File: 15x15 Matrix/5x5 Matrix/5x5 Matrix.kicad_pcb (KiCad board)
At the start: 2 copper layers, 127.8 x 152.5 mm, 111 parts, among them J1 Conn_01x02, SW1 SWP, SW10 SWP, SW11 SWP, SW12 SWP, SW13 SWP, SW14 SWP, SW15 SWP, SW16 SWP, SW17 SWP, SW18 SWP, SW19 SWP, SW2 SWP, SW20 SWP, SW21 SWP, SW22 SWP, SW23 SWP, SW24 SWP, SW25 SWP, SW3 SWP, SW4 SWP, SW5 SWP, SW6 SWP, SW7 SWP, SW8 SWP, SW9 SWP, U1 MCP23017-E/SO, U2 74AHCT1G125

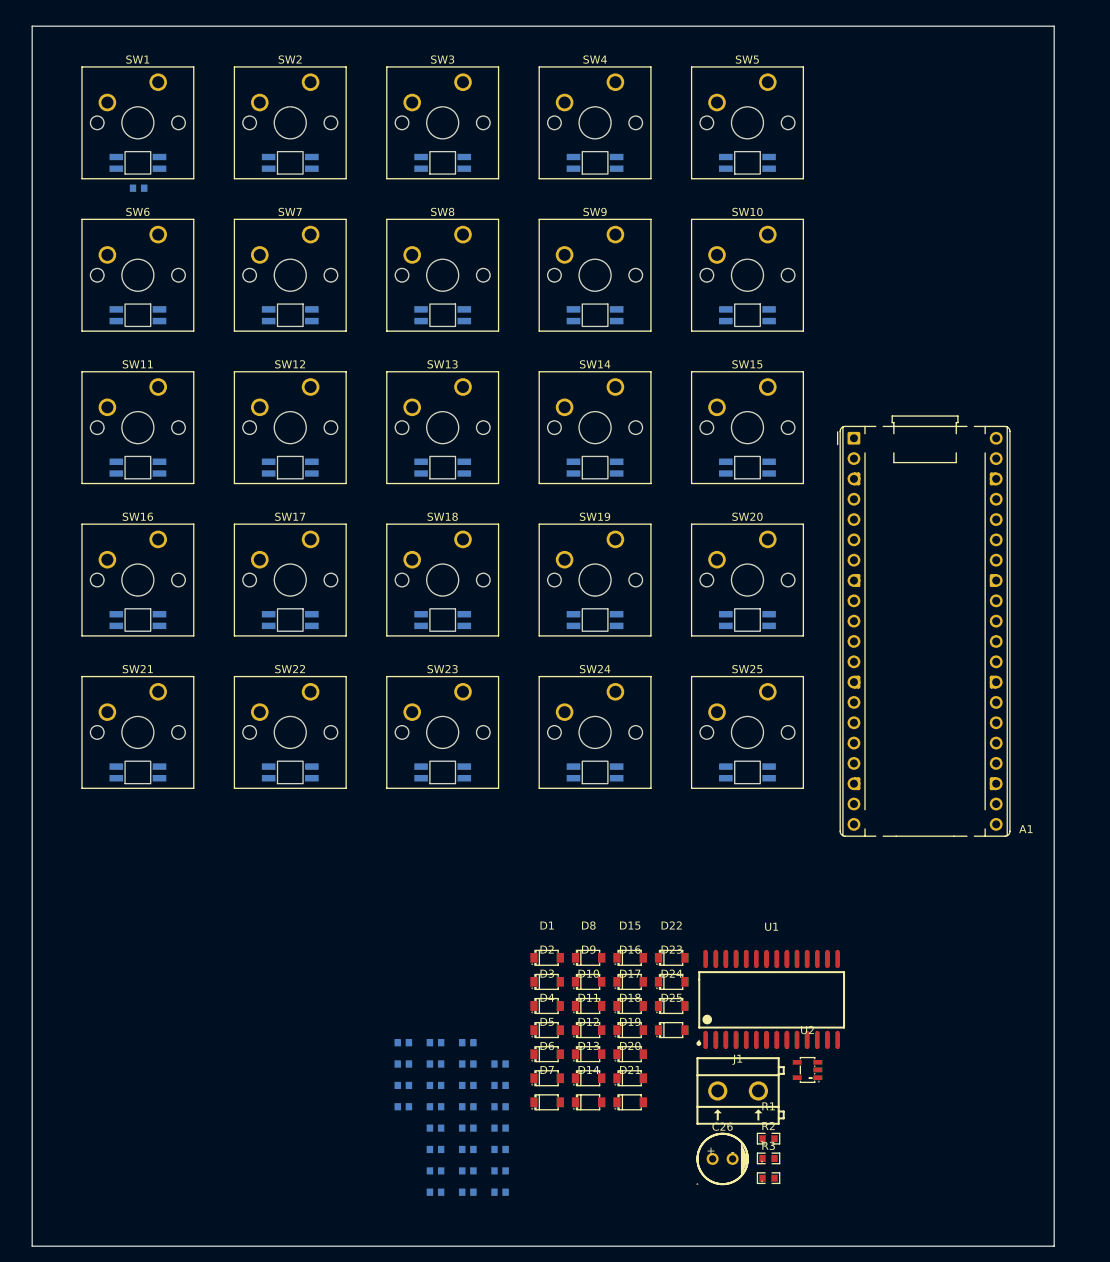
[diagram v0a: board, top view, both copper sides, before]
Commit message: 5x5 Ready for 1 sided printing
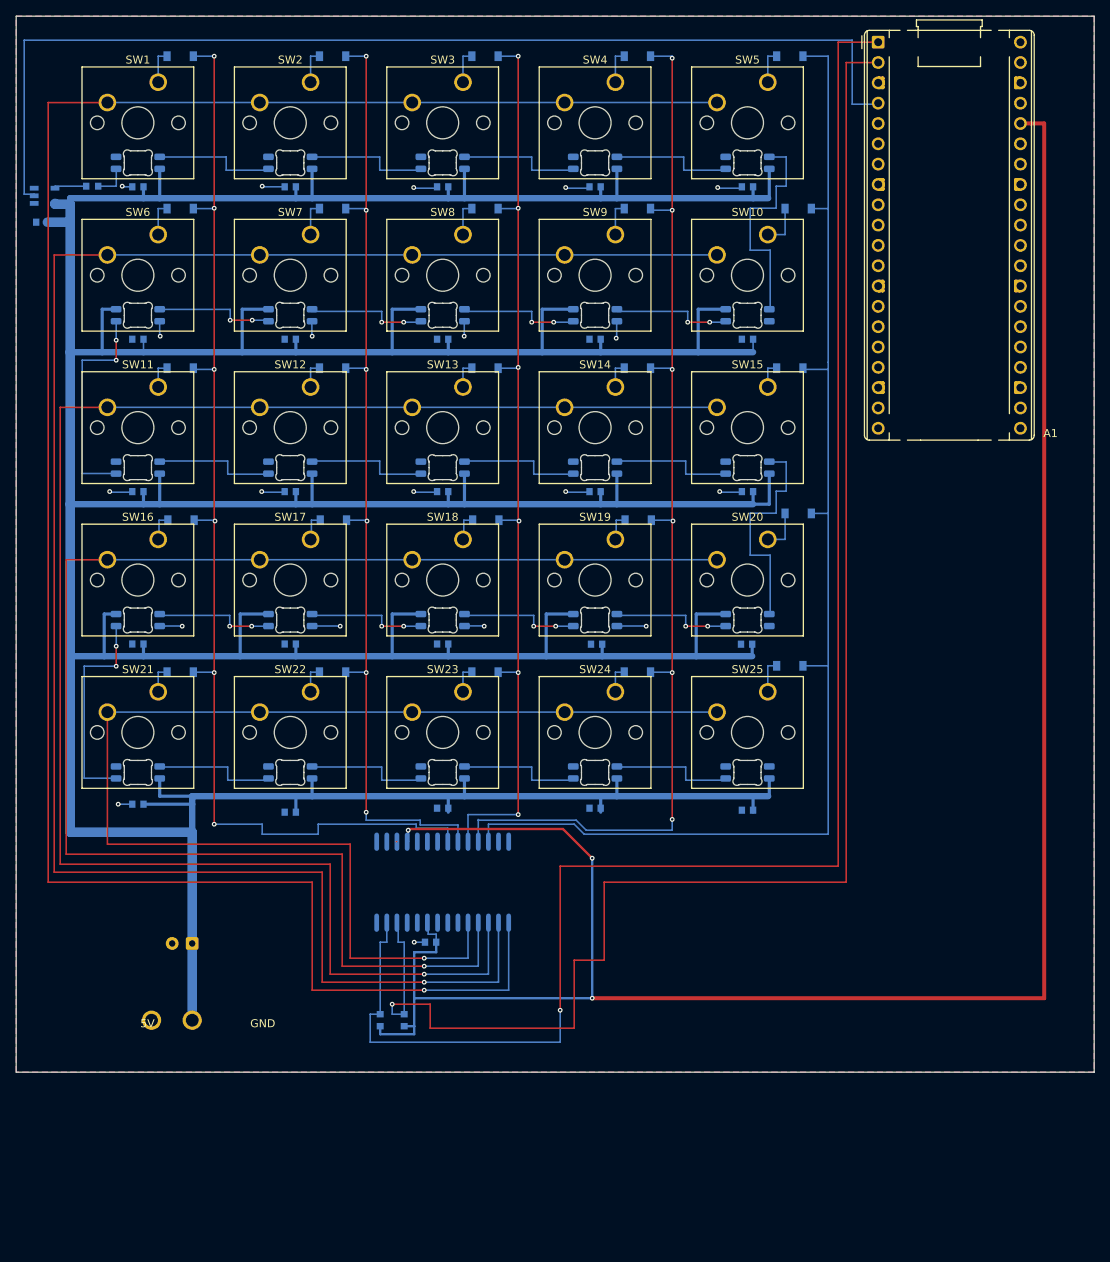
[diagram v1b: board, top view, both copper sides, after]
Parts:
- removed CPI1: 100nF, footprints:C14663_C0603
- C26: footprint footprints:C49304896_CAP-TH_BD6_3-P2_50-D0_5-FD -> Capacitor_THT:CP_Radial_D6.3mm_P2.50mm; moved to B.Cu
- D1, D10, D11, D12, D13, D14, D15, D16, D17, D18, D19, D2, D20, D21, D22, D23, D24, D25, D3, D4, D5, D6, D7, D8, D9, J1, R1, R2, R3, U1, U2: moved to B.Cu
- D26, D27, D28, D29, D30, D31, D32, D33, D34, D35, D36, D37, D38, D39, D40, D41, D42, D43, D44, D45, D46, D47, D48, D49, D50: footprint footprints:C5149201_LED-SMD_4P-L3_2-W2_8-LS5_9_SK6812MINI-E -> LED_SMD:LED_SK6812MINI-E_3.2x2.8mm_P1.5mm_ReverseMount
- moved R3 150.1 mm to (21.8, 43.0), turned to 180 degrees
- moved U2 145.0 mm to (15.8, 44.2), turned to 180 degrees
- moved D5 128.4 mm to (109.0, 26.8), turned to 180 degrees
- moved D4 122.3 mm to (89.9, 26.8), turned to 180 degrees
- moved D1 121.7 mm to (32.8, 26.8), turned to 180 degrees
- moved C5 121.7 mm to (103.7, 43.1)
- moved D3 119.0 mm to (70.8, 26.8), turned to 180 degrees
- moved D2 118.8 mm to (51.8, 26.8), turned to 180 degrees
- moved D6 118.0 mm to (32.8, 45.8), turned to 180 degrees
- moved C4 115.6 mm to (84.6, 43.1)
- moved D7 114.9 mm to (51.8, 45.8), turned to 180 degrees
- moved C27 114.5 mm to (15.4, 47.5), turned to 0 degrees
- moved C2 112.7 mm to (46.5, 43.1)
- moved C3 112.5 mm to (65.6, 43.1)
- moved C8 106.9 mm to (65.6, 62.1)
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- renumbered CPI2 to C28
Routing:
- net /5V: track 0.00 -> 727.9 mm
- net /ROW0: track 0.00 -> 260.6 mm, vias 0 -> 1
- net /3V3: track 0.00 -> 259.1 mm, vias 0 -> 3
- net /ROW1: track 0.00 -> 236.7 mm, vias 0 -> 1
- net /ROW2: track 0.00 -> 212.9 mm, vias 0 -> 1
- net /I2C_SDA: track 0.00 -> 205.6 mm, vias 0 -> 1
- net /I2C_SCL: track 0.00 -> 199.6 mm, vias 0 -> 1
- net /ROW3: track 0.00 -> 189.1 mm, vias 0 -> 1
- net /ROW4: track 0.00 -> 156.5 mm, vias 0 -> 1
- net /COL4: track 0.00 -> 156.1 mm
- net /COL0: track 0.00 -> 143.0 mm, vias 0 -> 6
- net /COL3: track 0.00 -> 138.0 mm, vias 0 -> 6
- net /GPIO2: track 0.00 -> 135.6 mm
- net /COL1: track 0.00 -> 122.5 mm, vias 0 -> 6
- net /COL2: track 0.00 -> 117.0 mm, vias 0 -> 6
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- added copper zone on B.Cu, net /GND
- added copper zone on F.Cu, net /GND
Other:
- board size 127.8 x 152.5 mm -> 134.8 x 132 mm
- board text added: "5V"
- board text added: "GND"
